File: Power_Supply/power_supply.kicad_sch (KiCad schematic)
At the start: 14 parts, among them J3 Conn_ARM_SWD_TagConnect, J6 Conn_01x04_Pin, SW1 SW_Push, U1 STM32F401RBTx, Y1 26MHz

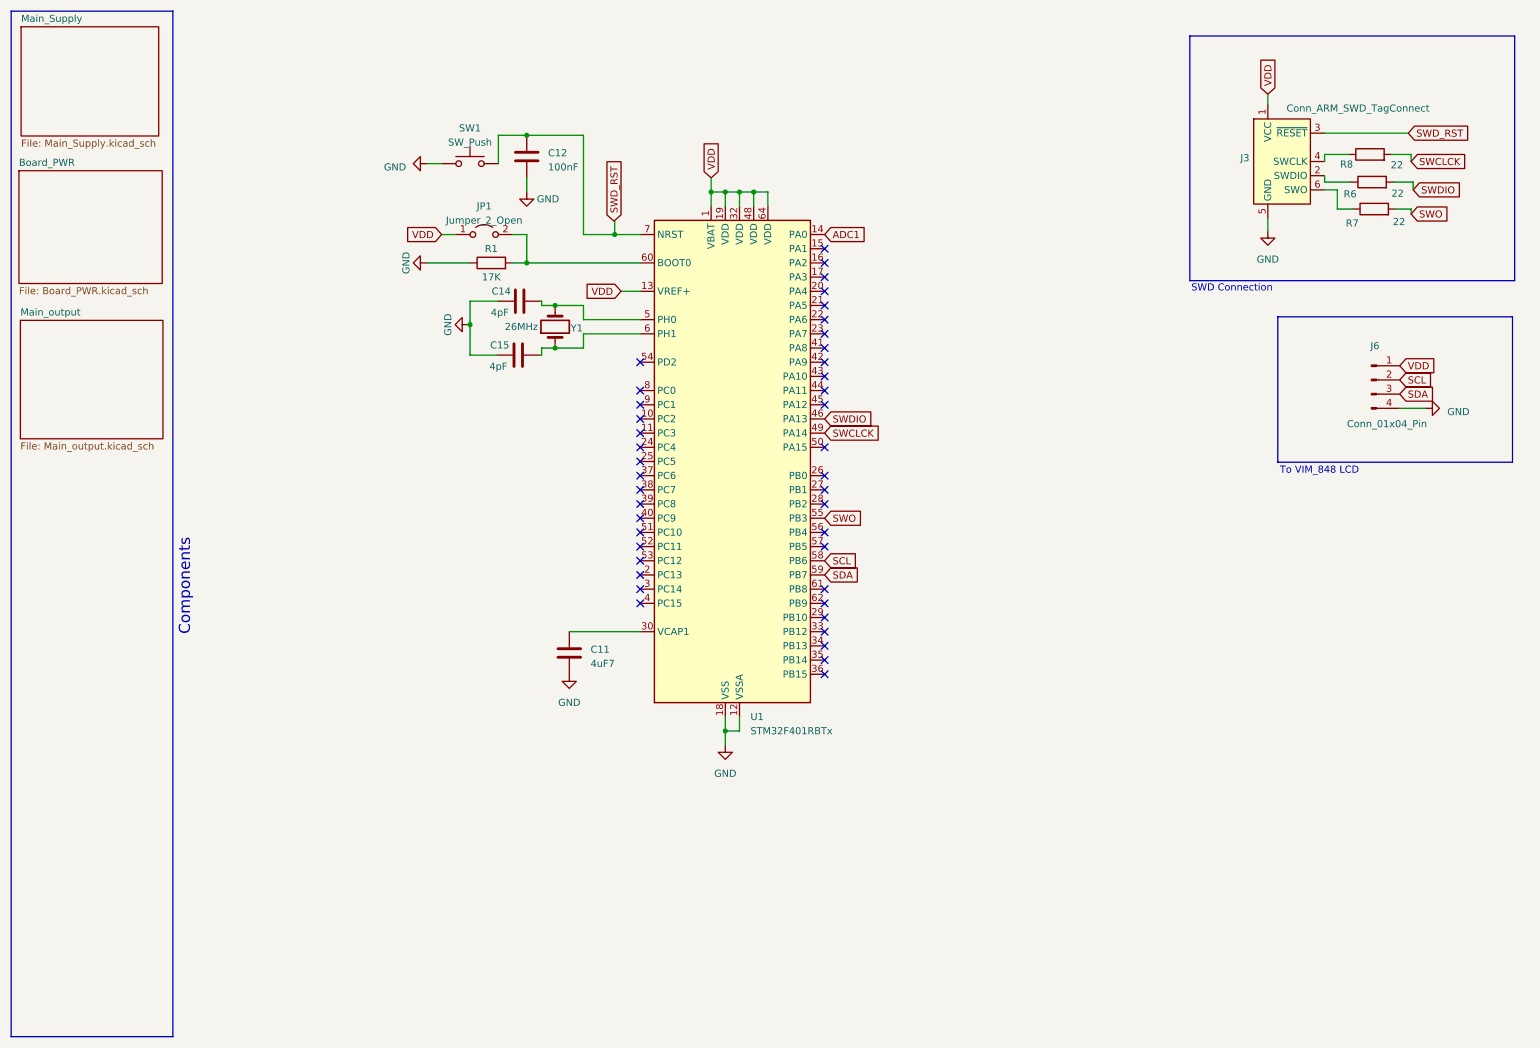
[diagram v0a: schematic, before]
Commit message: Updated Schematic and VIM878
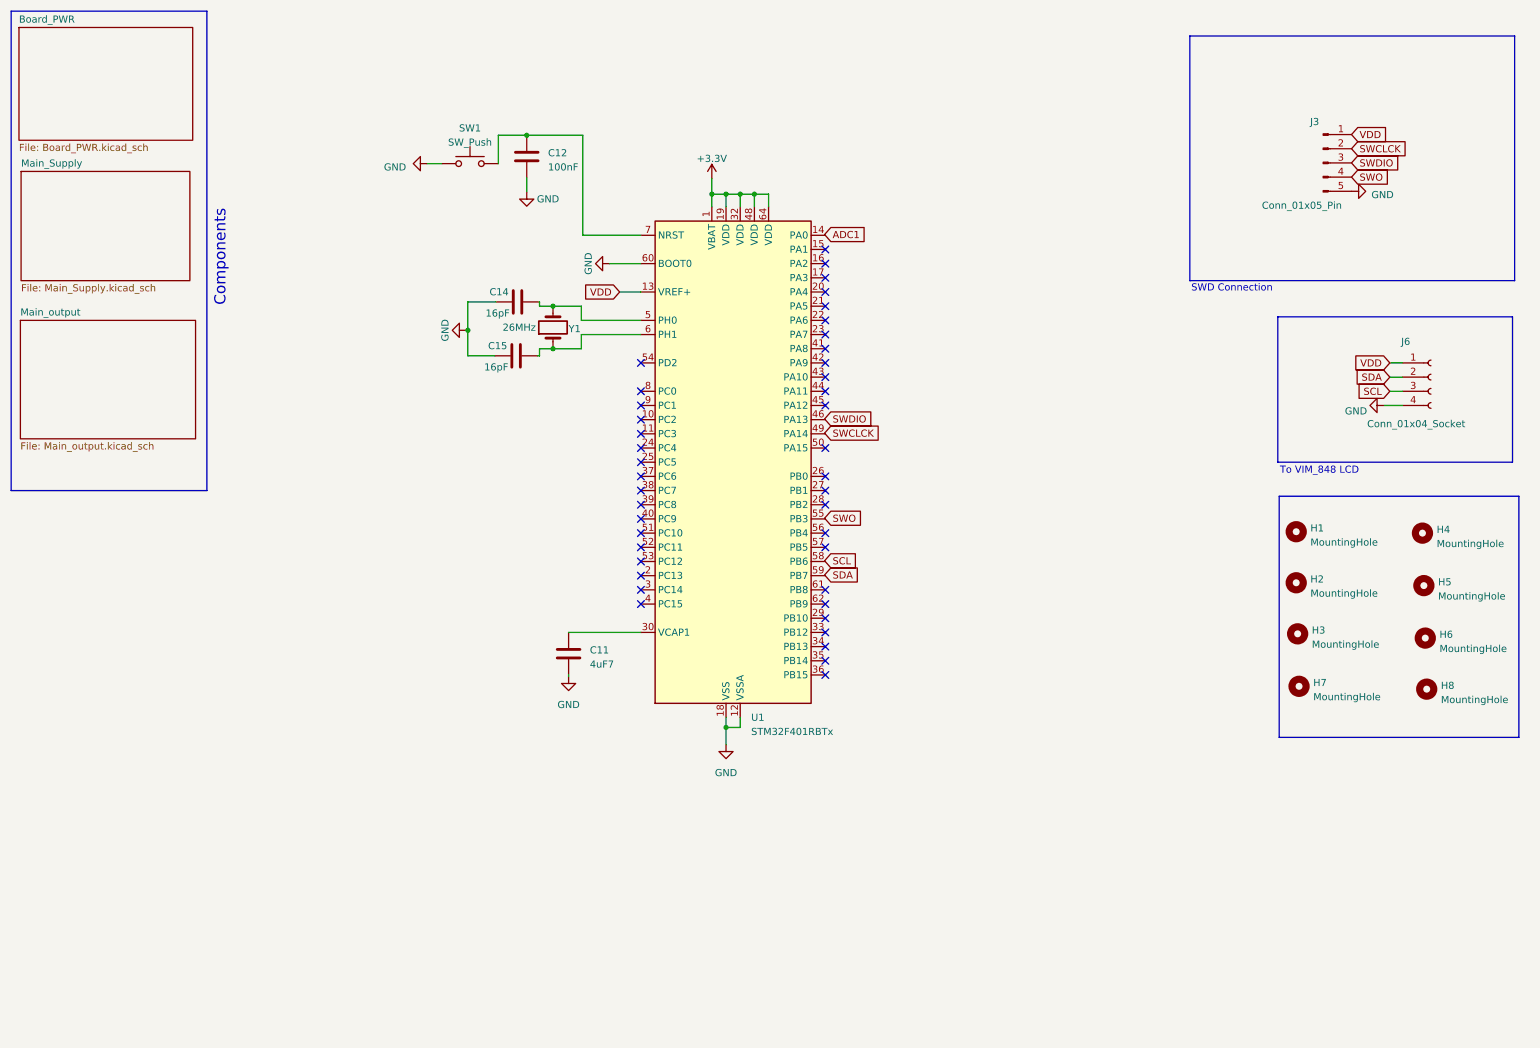
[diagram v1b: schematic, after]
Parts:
- removed J3: Conn_ARM_SWD_TagConnect, Connector:Tag-Connect_TC2030-IDC-NL_2x03_P1.27mm_Vertical, symbol Connector:Conn_ARM_SWD_TagConnect_TC2030-NL
- removed J6: Conn_01x04_Pin, symbol Connector:Conn_01x04_Pin
- removed JP1: Jumper_2_Open, TestPoint:TestPoint_Bridge_Pitch2.54mm_Drill0.7mm, symbol Jumper:Jumper_2_Open
- removed R1: 17K, symbol Device:R
- removed R6, R7, R8: 22, symbol Device:R
- added H1, H2, H3, H4: MountingHole, MountingHole:MountingHole_2.1mm, symbol Mechanical:MountingHole
- added H5, H6, H7, H8: MountingHole, MountingHole:MountingHole_3.2mm_M3, symbol Mechanical:MountingHole
- added J3: Conn_01x05_Pin, Connector_JST:JST_EH_B5B-EH-A_1x05_P2.50mm_Vertical, symbol Connector:Conn_01x05_Pin
- added J6: Conn_01x04_Socket, Connector_JST:JST_EH_B4B-EH-A_1x04_P2.50mm_Vertical, symbol Connector:Conn_01x04_Socket
- C11: footprint (none) -> Capacitor_SMD:C_0603_1608Metric
- C12: footprint (none) -> Capacitor_SMD:C_0402_1005Metric
- C14, C15: value 4pF -> 16pF; footprint (none) -> Capacitor_SMD:C_0402_1005Metric
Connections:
- net GND: now also U1.60 (BOOT0), J3.5 (Pin_5), J6.4 (Pin_4)
- net SCL: now also J6.3 (Pin_3)
- net SDA: now also J6.2 (Pin_2)
- net SWCLCK: now also J3.2 (Pin_2)
- net SWDIO: now also J3.3 (Pin_3)
- net SWO: now also J3.4 (Pin_4)
- net VDD: now also J3.1 (Pin_1), J6.1 (Pin_1); no longer U1.1 (VBAT), U1.19 (VDD), U1.32 (VDD), U1.48 (VDD), U1.64 (VDD)
- net SWD_RST: no longer names the net of C12.1, SW1.2, U1.7 (NRST)
- new net +3.3V: U1.1 (VBAT), U1.19 (VDD), U1.32 (VDD), U1.48 (VDD), U1.64 (VDD)
